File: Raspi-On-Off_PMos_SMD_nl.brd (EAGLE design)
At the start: 52 x 28 mm, 33 parts, among them IC1 74AUC1G17, T1 FDC6327C, T2 FDC6327C, T3 IRLML2803, T4 IRF7416, T5 IRLML0030, X1 MKDSN1,5/2-5,08

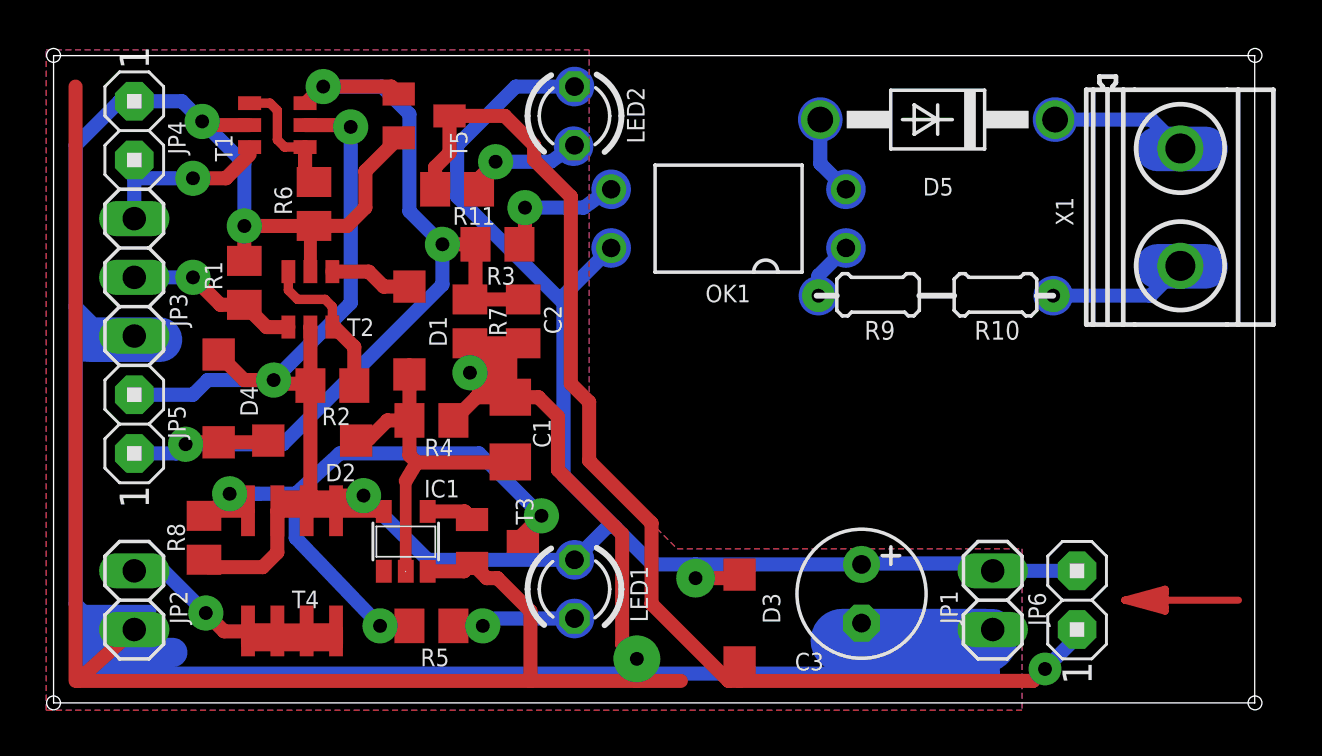
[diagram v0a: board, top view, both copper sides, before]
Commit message: Add files via upload
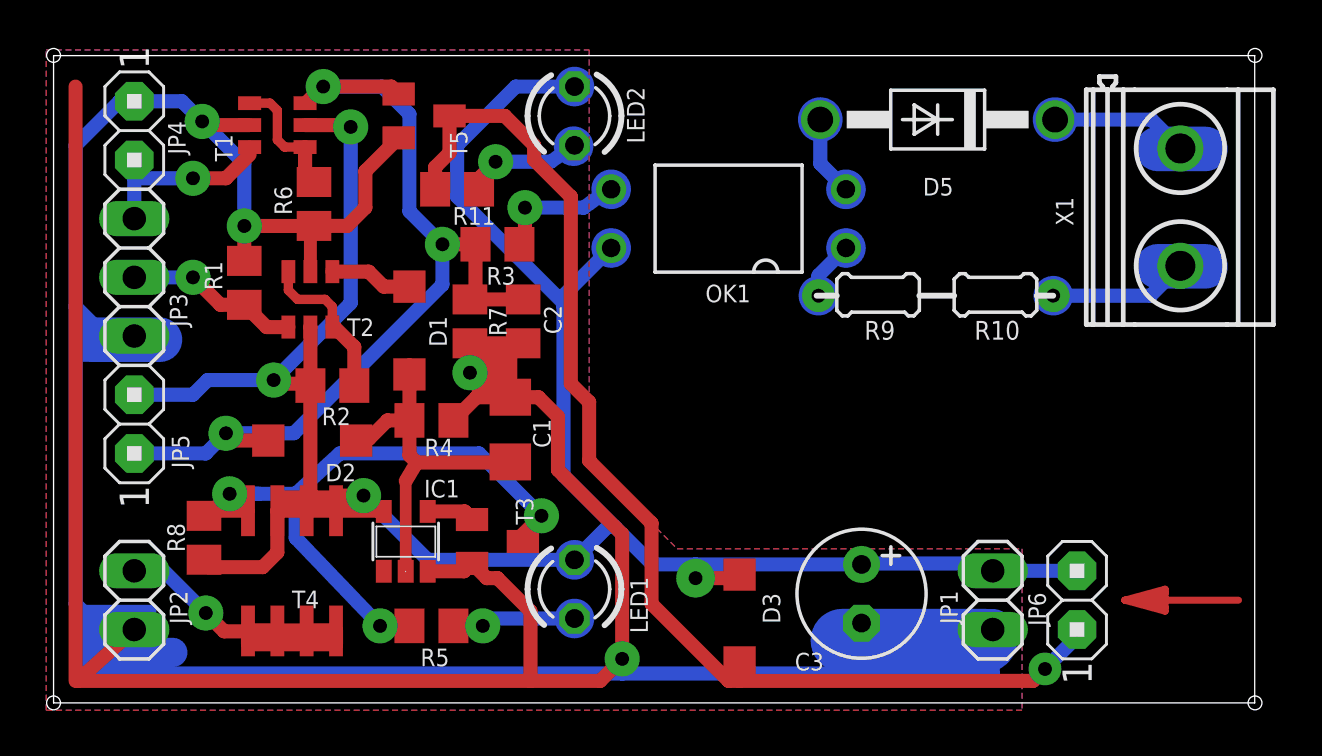
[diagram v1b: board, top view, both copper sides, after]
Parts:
- removed D4: SS12, diode2:SOD123
- T3: value IRLML2803 -> BSS123
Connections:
- net +5V: no longer D4.C
- net N$8: no longer D4.A
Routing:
- net GND: track 196.4 -> 193.0 mm
- net +5V: track 111.9 -> 109.1 mm
- net N$8: track 42.9 -> 41.2 mm
